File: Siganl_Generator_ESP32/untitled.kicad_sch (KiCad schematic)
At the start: 5 parts, among them J3 USB_C_Receptacle_PowerOnly_6P

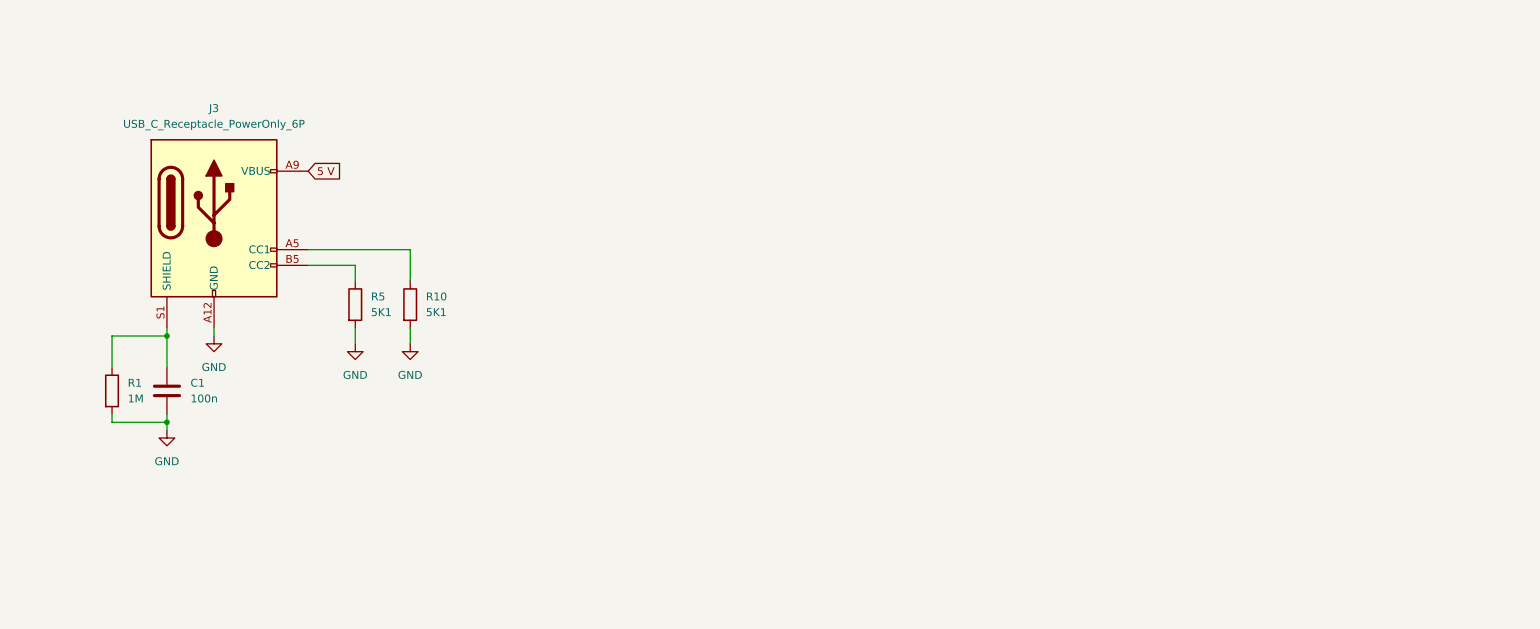
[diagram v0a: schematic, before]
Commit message: update
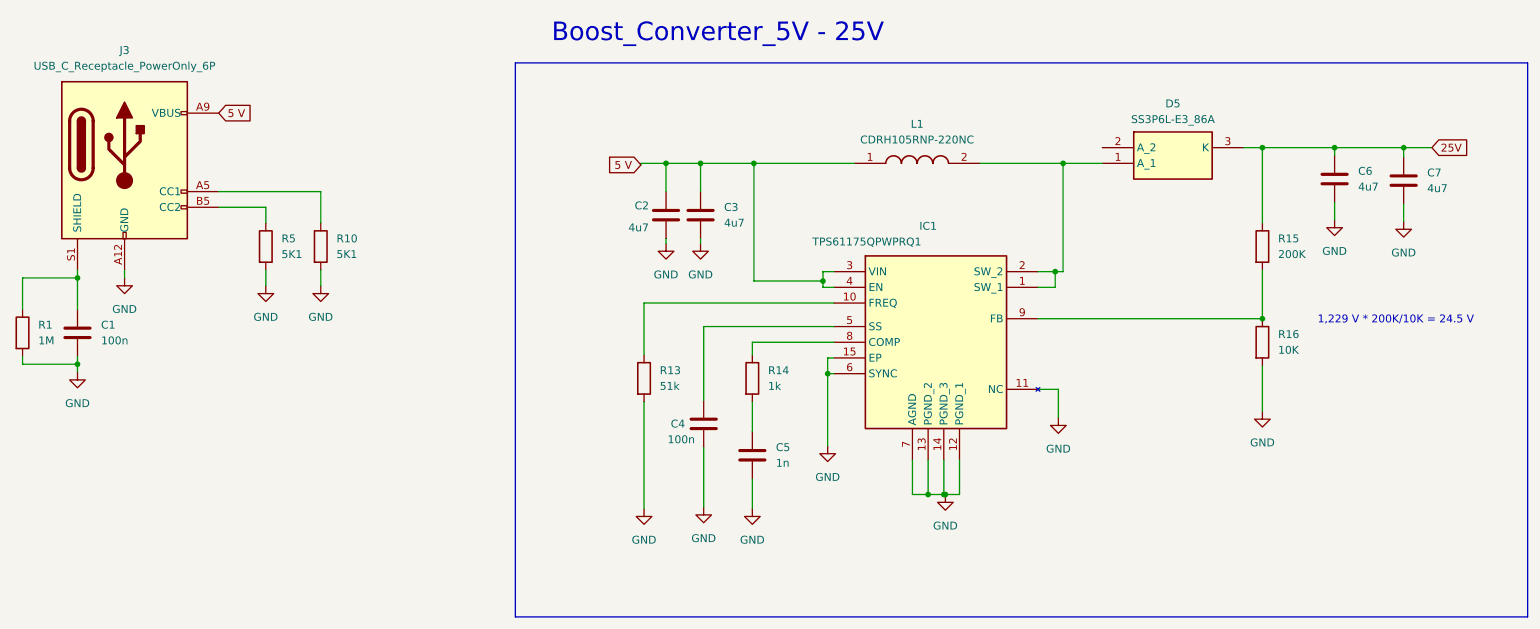
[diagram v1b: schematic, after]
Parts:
- added C2, C3, C6, C7: 4u7, Capacitor_SMD:C_1206_3216Metric_Pad1.33x1.80mm_HandSolder, symbol Device:C
- added C4: 100n, Capacitor_SMD:C_0603_1608Metric_Pad1.08x0.95mm_HandSolder, symbol Device:C
- added C5: 1n, Capacitor_SMD:C_0603_1608Metric_Pad1.08x0.95mm_HandSolder, symbol Device:C
- added D5: SS3P6L-E3_86A, Amjad_lib:SS3P6LE386A, symbol Amjads_Lib:SS3P6L-E3_86A
- added IC1: TPS61175QPWPRQ1, Amjad_lib:SOP65P640X120-15N, symbol Amjads_Lib:TPS61175QPWPRQ1
- added L1: CDRH105RNP-220NC, Amjad_lib:INDPM102100X510N_Spule, symbol Amjads_Lib:CDRH105RNP-220NC
- added R13: 51k, Resistor_SMD:R_0603_1608Metric_Pad0.98x0.95mm_HandSolder, symbol Device:R
- added R14: 1k, Resistor_SMD:R_0603_1608Metric_Pad0.98x0.95mm_HandSolder, symbol Device:R
- added R15: 200K, Resistor_SMD:R_0603_1608Metric_Pad0.98x0.95mm_HandSolder, symbol Device:R
- added R16: 10K, Resistor_SMD:R_0603_1608Metric_Pad0.98x0.95mm_HandSolder, symbol Device:R
- R10, R5: footprint Resistor_SMD:R_1206_3216Metric -> Resistor_SMD:R_0603_1608Metric_Pad0.98x0.95mm_HandSolder
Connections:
- net 5 V: now also C2.1, C3.1, IC1.3 (VIN), IC1.4 (EN), L1.1
- net GND: now also C2.2, C3.2, C4.2, C5.2, C6.2, C7.2, IC1.11 (NC), IC1.12 (PGND_1), IC1.13 (PGND_2), IC1.14 (PGND_3), IC1.15 (EP), IC1.6 (SYNC), IC1.7 (AGND), R13.2, R16.2
- new net: IC1.10 (FREQ), R13.1
- new net: D5.1 (A_1), IC1.1 (SW_1), IC1.2 (SW_2), L1.2
- new net: C4.1, IC1.5 (SS)
- new net: IC1.8 (COMP), R14.1
- new net: IC1.9 (FB), R15.2, R16.1
- new net: C5.1, R14.2
- new net 25V: C6.1, C7.1, D5.3 (K), R15.1
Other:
- note added: "1,229 V * 200K/10K = 24.5 V"
- note added: "Boost_Converter_5V - 25V"
- moved on the sheet: C1, J3, R1, R10, R5
